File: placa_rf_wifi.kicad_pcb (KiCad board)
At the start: 2 copper layers, 7 parts

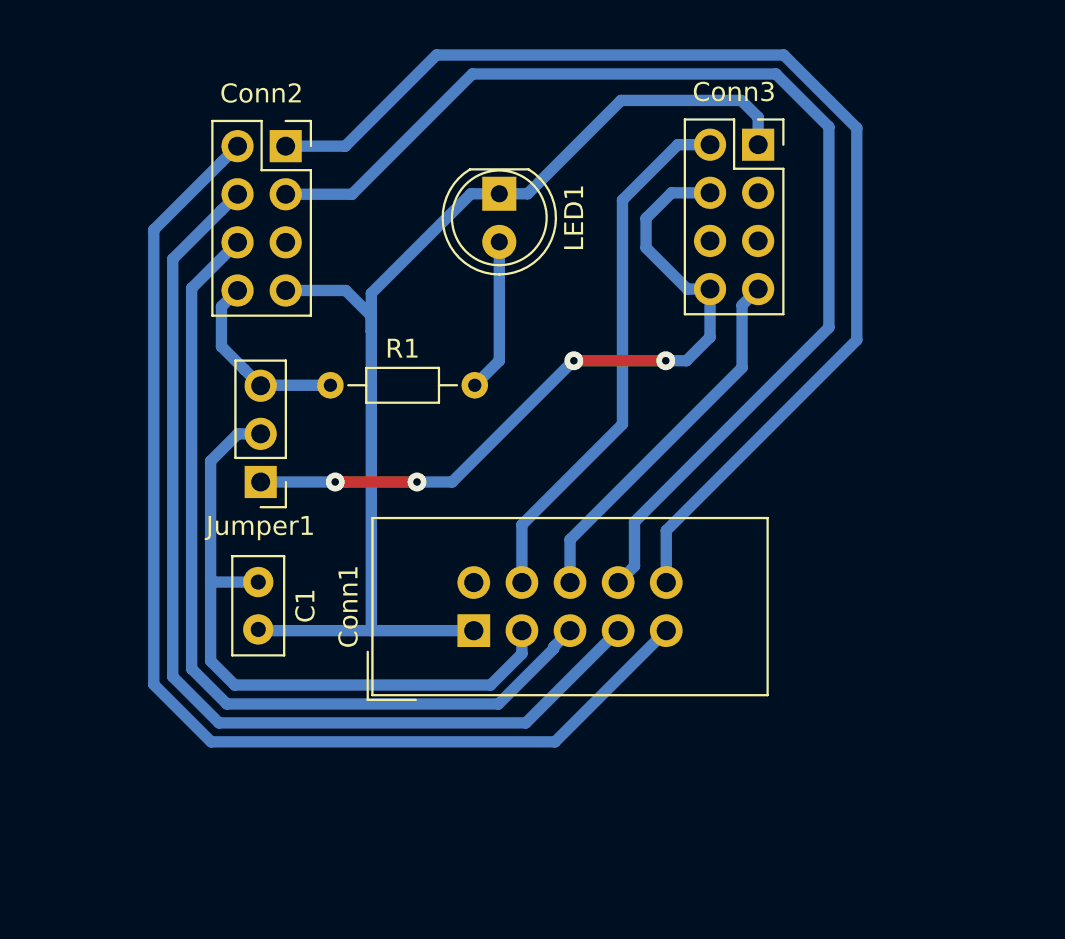
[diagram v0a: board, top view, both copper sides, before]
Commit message: Placa completa, ordenada, doble capa
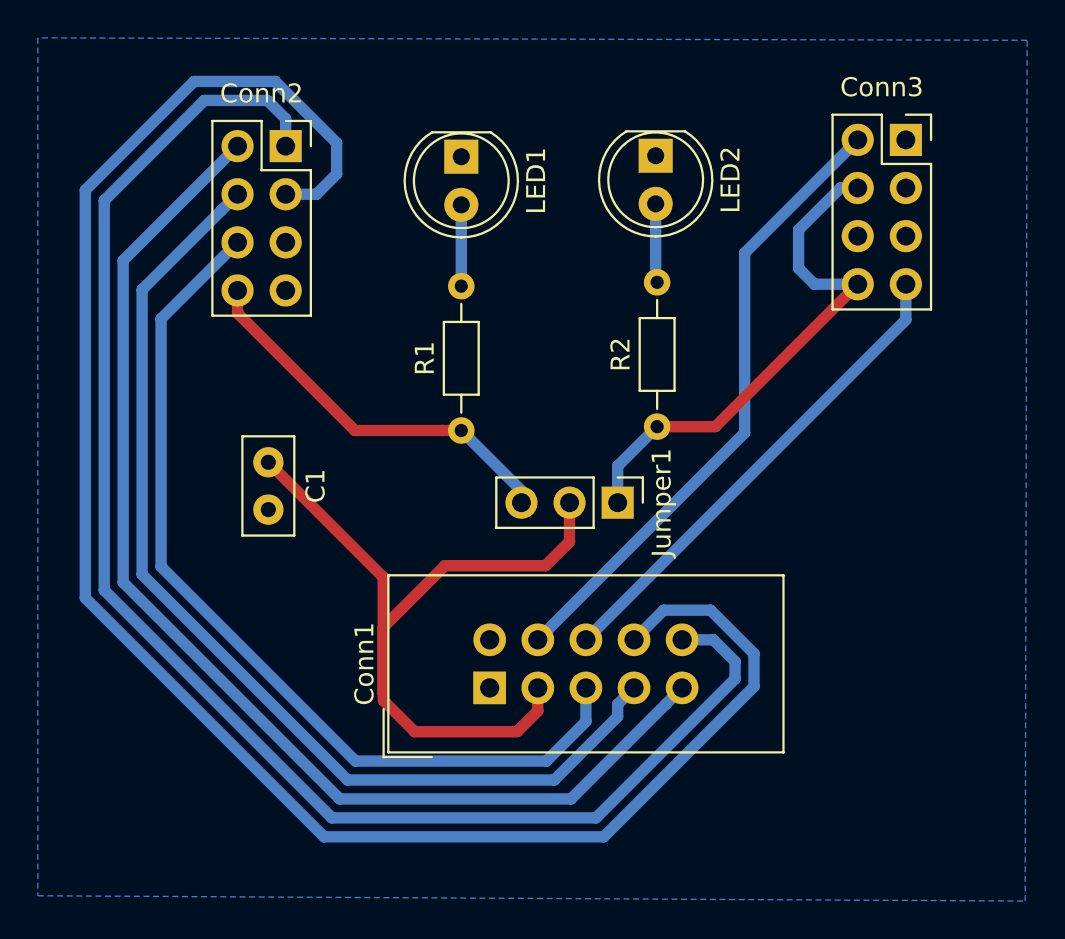
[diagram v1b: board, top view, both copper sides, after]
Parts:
- added LED2: D_Wifi, LED_THT:LED_D5.0mm, F.Cu at (149.0, 75.7)
- added R2: R_Wifi, Resistor_THT:R_Axial_DIN0204_L3.6mm_D1.6mm_P7.62mm_Horizontal, F.Cu at (149.1, 90.0)
- moved Jumper1 18.9 mm to (147.0, 94.0), turned to 270 degrees
- moved Conn3 7.80 mm to (162.2, 74.9)
- moved R1 7.31 mm to (138.7, 90.2), turned to 90 degrees
- moved C1 6.35 mm to (128.5, 91.9)
- moved Conn1 3.14 mm to (140.2, 103.8)
- moved LED1 2.80 mm to (138.7, 75.7)
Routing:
- net GND: track 61.6 -> 0.00 mm
- net SCK: track 61.1 -> 96.8 mm
- net MISO: track 61.9 -> 79.7 mm
- net VccWifi: track 39.2 -> 28.1 mm, vias 4 -> 0
- net VccRF: track 9.93 -> 20.7 mm
- net +3V3: track 35.2 -> 42.9 mm
- net RX: track 19.6 -> 25.8 mm
- net TX: track 28.2 -> 33.4 mm
- net Net-(LED2-Pad2): track 0.00 -> 4.17 mm
- net Net-(LED1-Pad2): track 8.11 -> 4.29 mm
- net CSN: track 45.9 -> 48.1 mm
- net MOSI: track 53.4 -> 55.0 mm
- net IRQ: track 61.0 -> 62.2 mm
- added copper zone on B.Cu, net GND
